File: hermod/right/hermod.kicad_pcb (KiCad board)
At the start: 2 copper layers, 154 x 149.2 mm, 164 parts, among them J1 USB_C_Receptacle_USB2.0, J2 Conn_01x05, J3 USB_C_Receptacle_USB2.0, Q1 AO3401A, Q2 MMUN2233LT1G, U1 STM32F072CBT6, U2 PRTR5V0U2X, U3 XC6206PxxxMR-Regulator_Linear, U4 CR2013-MI2120, U5 TXB0101

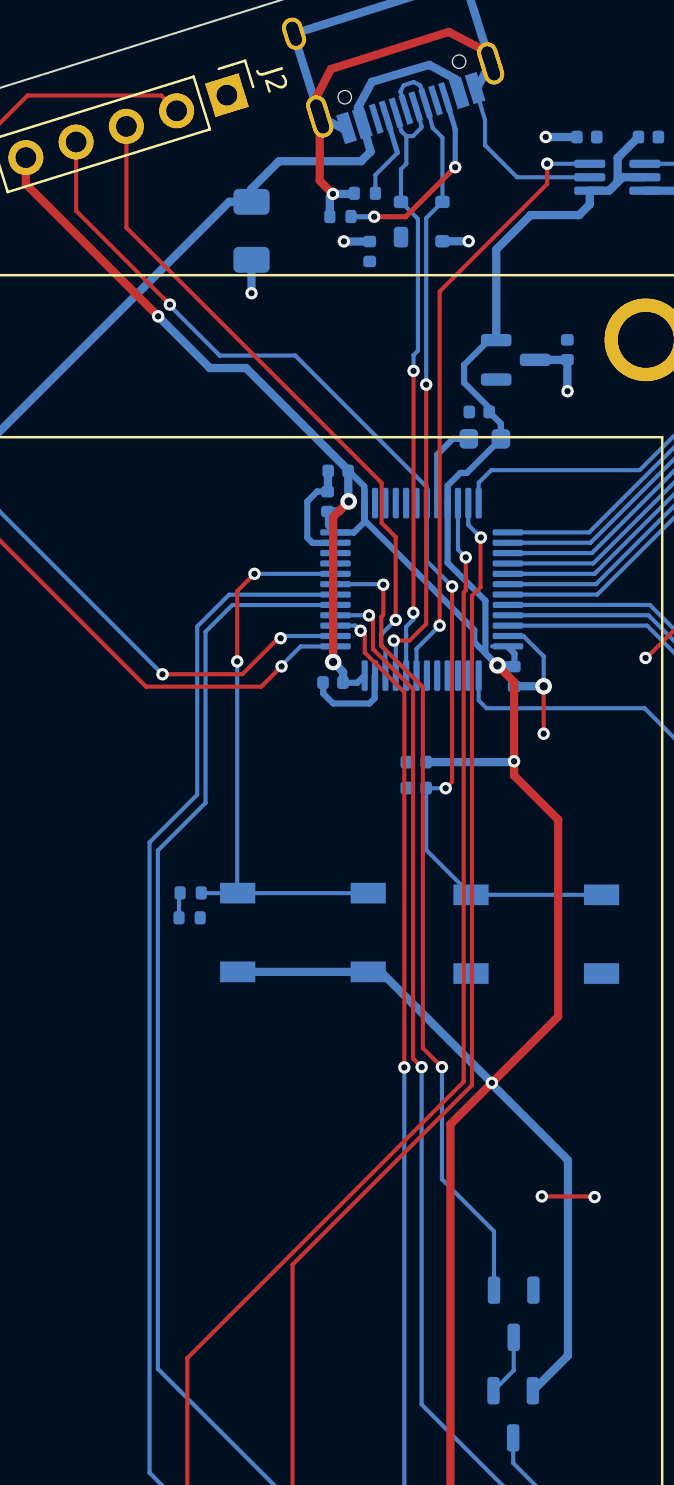
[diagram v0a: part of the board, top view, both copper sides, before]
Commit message: Finished routing
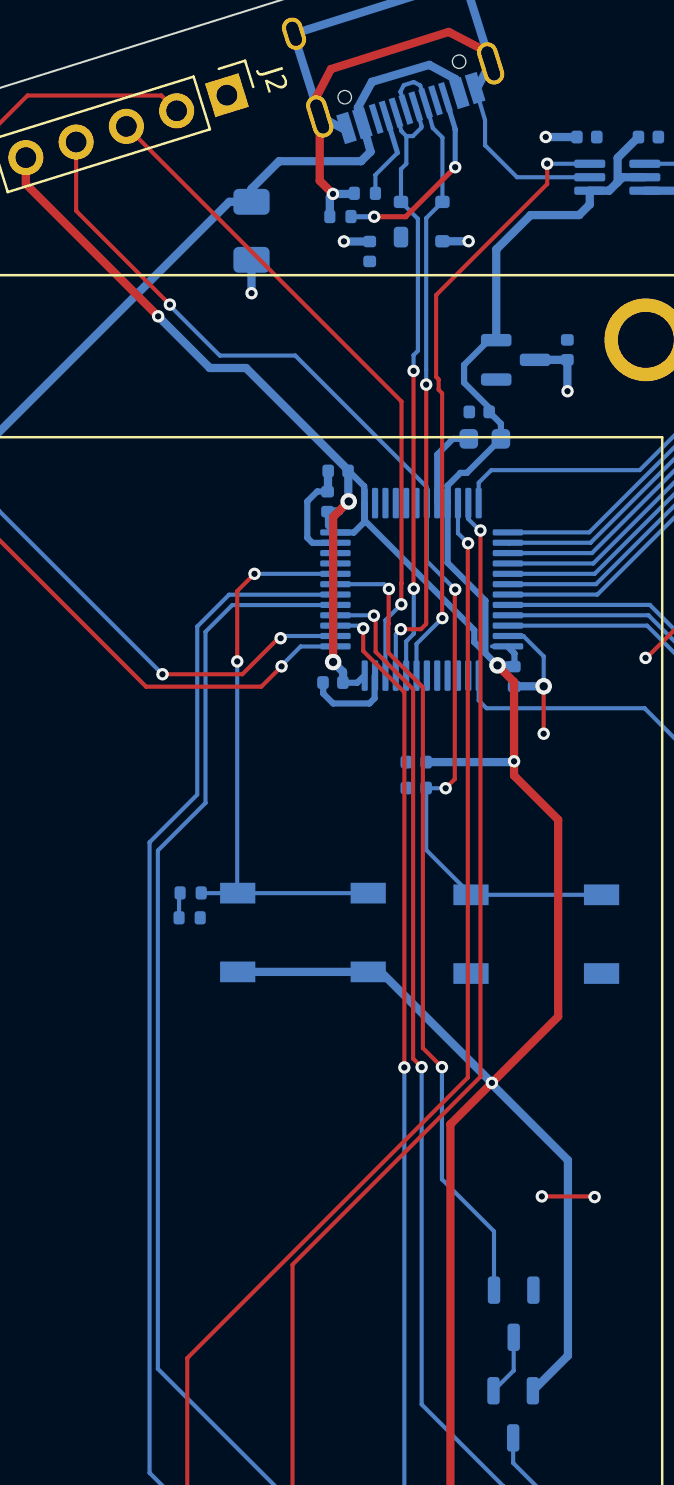
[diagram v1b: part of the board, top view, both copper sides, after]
